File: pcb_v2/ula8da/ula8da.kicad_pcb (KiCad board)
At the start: 2 copper layers, 66.6 x 123.8 mm, 28 parts, among them J1 addr_decoder, J2 Conn_01x07, J3 Conn_01x07, J4 Conn_01x07, J5 Conn_01x07, Q1 BC548, U1 74LS138, U2 74HC238, U3 74HC238, U4 74HC238, U5 74LS04, U6 74LS244, U7 74LS04, U8 MC14495P, U9 SA39-11EWA

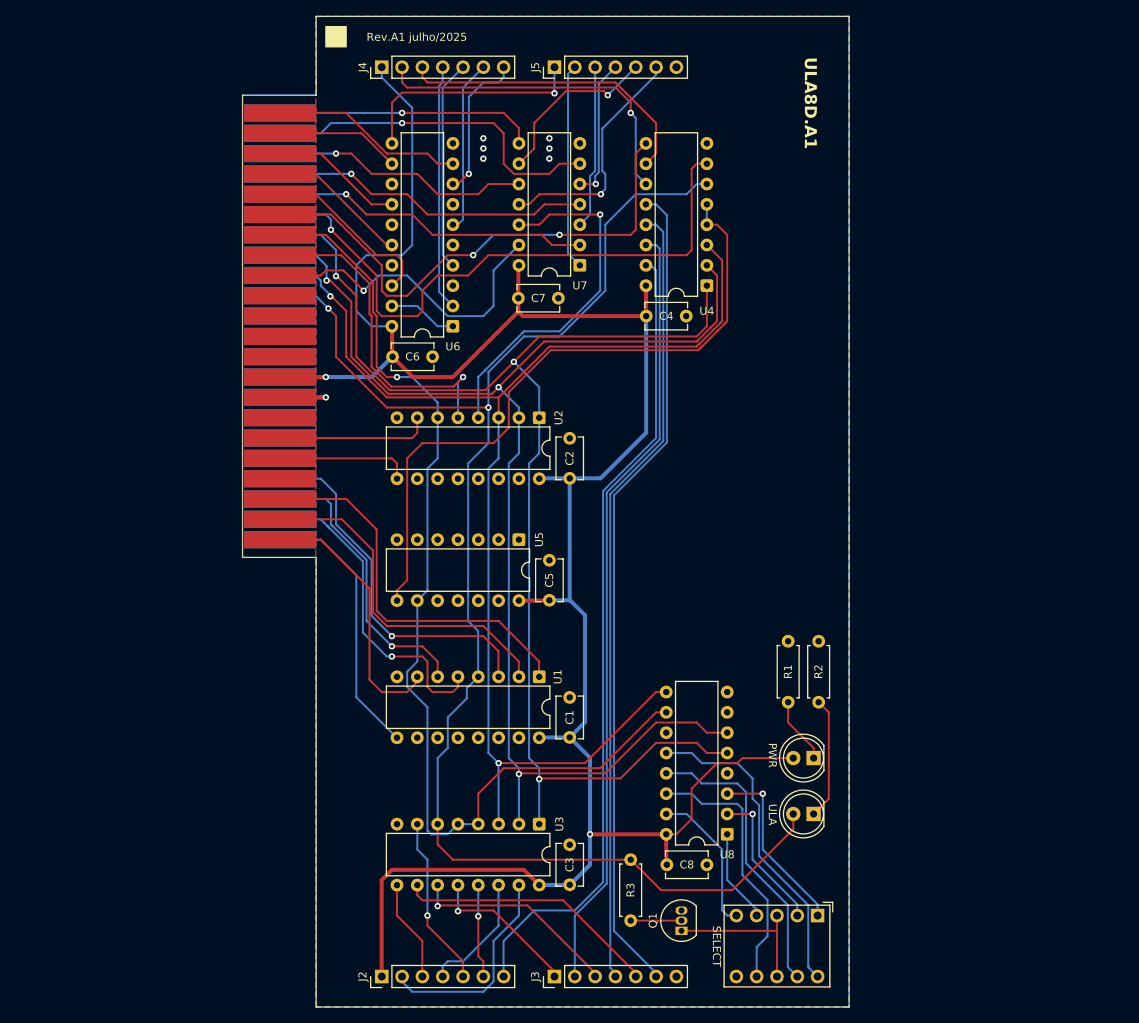
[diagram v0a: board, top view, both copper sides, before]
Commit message: PCB concluída
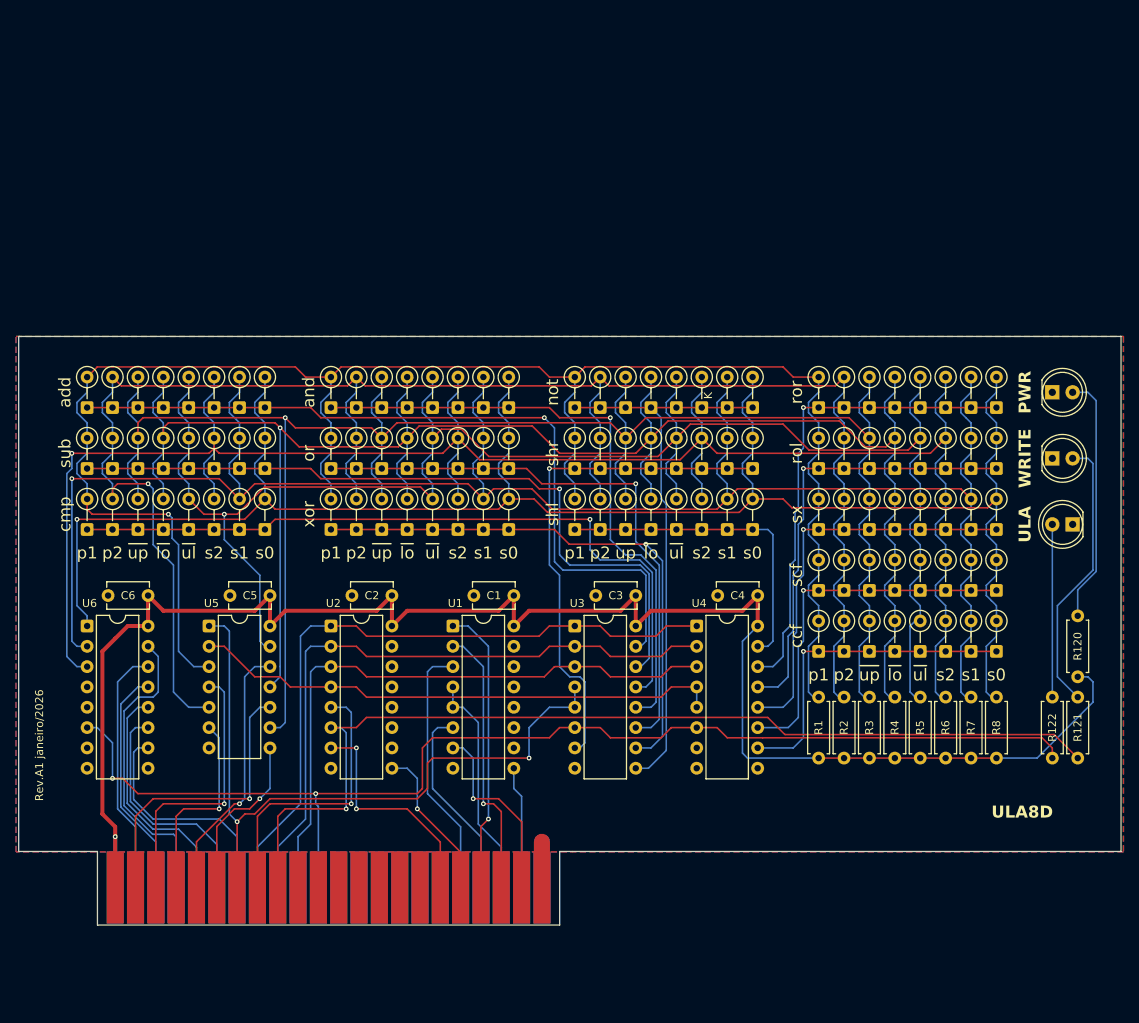
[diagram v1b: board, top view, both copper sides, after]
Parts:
- removed C7, C8: 100nF, Capacitor_THT:C_Disc_D5.1mm_W3.2mm_P5.00mm
- removed J2, J3, J4, J5: Conn_01x07, Connector_PinHeader_2.54mm:PinHeader_1x07_P2.54mm_Vertical
- removed Q1: BC548, Package_TO_SOT_THT:TO-92_Inline
- removed U7: 74LS04, Package_DIP:DIP-14_W7.62mm
- removed U8: MC14495P, Package_DIP:DIP-16_W7.62mm
- removed U9: SA39-11EWA, Display_7Segment:Sx39-1xxxxx
- added D10: 1N4148, Diode_THT:D_DO-35_SOD27_P3.81mm_Vertical_KathodeUp, F.Cu at (45.1, 88.9)
- added D100: 1N4148, Diode_THT:D_DO-35_SOD27_P3.81mm_Vertical_KathodeUp, F.Cu at (142.9, 104.1)
- added D101: 1N4148, Diode_THT:D_DO-35_SOD27_P3.81mm_Vertical_KathodeUp, F.Cu at (146.1, 104.1)
- added D102: 1N4148, Diode_THT:D_DO-35_SOD27_P3.81mm_Vertical_KathodeUp, F.Cu at (149.2, 104.1)
- added D103: 1N4148, Diode_THT:D_DO-35_SOD27_P3.81mm_Vertical_KathodeUp, F.Cu at (152.4, 104.1)
- added D104: 1N4148, Diode_THT:D_DO-35_SOD27_P3.81mm_Vertical_KathodeUp, F.Cu at (155.6, 104.1)
- added D105: 1N4148, Diode_THT:D_DO-35_SOD27_P3.81mm_Vertical_KathodeUp, F.Cu at (133.3, 111.8)
- added D106: 1N4148, Diode_THT:D_DO-35_SOD27_P3.81mm_Vertical_KathodeUp, F.Cu at (136.5, 111.8)
- added D107: 1N4148, Diode_THT:D_DO-35_SOD27_P3.81mm_Vertical_KathodeUp, F.Cu at (139.7, 111.8)
- added D108: 1N4148, Diode_THT:D_DO-35_SOD27_P3.81mm_Vertical_KathodeUp, F.Cu at (142.9, 111.8)
- added D109: 1N4148, Diode_THT:D_DO-35_SOD27_P3.81mm_Vertical_KathodeUp, F.Cu at (146.1, 111.8)
- added D11: 1N4148, Diode_THT:D_DO-35_SOD27_P3.81mm_Vertical_KathodeUp, F.Cu at (48.3, 88.9)
- added D110: 1N4148, Diode_THT:D_DO-35_SOD27_P3.81mm_Vertical_KathodeUp, F.Cu at (149.2, 111.8)
- added D111: 1N4148, Diode_THT:D_DO-35_SOD27_P3.81mm_Vertical_KathodeUp, F.Cu at (152.4, 111.8)
- added D112: 1N4148, Diode_THT:D_DO-35_SOD27_P3.81mm_Vertical_KathodeUp, F.Cu at (155.6, 111.8)
- added D12: 1N4148, Diode_THT:D_DO-35_SOD27_P3.81mm_Vertical_KathodeUp, F.Cu at (51.4, 88.9)
- added D120: LED, LED_THT:LED_D5.0mm, F.Cu at (162.6, 79.4)
- added D121: LED, LED_THT:LED_D5.0mm, F.Cu at (162.6, 87.6)
- added D122: LED, LED_THT:LED_D5.0mm, F.Cu at (165.1, 95.9)
- added D13: 1N4148, Diode_THT:D_DO-35_SOD27_P3.81mm_Vertical_KathodeUp, F.Cu at (54.6, 88.9)
- added D14: 1N4148, Diode_THT:D_DO-35_SOD27_P3.81mm_Vertical_KathodeUp, F.Cu at (57.8, 88.9)
- added D15: 1N4148, Diode_THT:D_DO-35_SOD27_P3.81mm_Vertical_KathodeUp, F.Cu at (61.0, 88.9)
- added D16: 1N4148, Diode_THT:D_DO-35_SOD27_P3.81mm_Vertical_KathodeUp, F.Cu at (64.1, 88.9)
- added D17: 1N4148, Diode_THT:D_DO-35_SOD27_P3.81mm_Vertical_KathodeUp, F.Cu at (41.9, 96.5)
- added D18: 1N4148, Diode_THT:D_DO-35_SOD27_P3.81mm_Vertical_KathodeUp, F.Cu at (45.1, 96.5)
- added D19: 1N4148, Diode_THT:D_DO-35_SOD27_P3.81mm_Vertical_KathodeUp, F.Cu at (48.3, 96.5)
- added D20: 1N4148, Diode_THT:D_DO-35_SOD27_P3.81mm_Vertical_KathodeUp, F.Cu at (51.4, 96.5)
- added D21: 1N4148, Diode_THT:D_DO-35_SOD27_P3.81mm_Vertical_KathodeUp, F.Cu at (54.6, 96.5)
- added D22: 1N4148, Diode_THT:D_DO-35_SOD27_P3.81mm_Vertical_KathodeUp, F.Cu at (57.8, 96.5)
- added D23: 1N4148, Diode_THT:D_DO-35_SOD27_P3.81mm_Vertical_KathodeUp, F.Cu at (61.0, 96.5)
- added D24: 1N4148, Diode_THT:D_DO-35_SOD27_P3.81mm_Vertical_KathodeUp, F.Cu at (64.1, 96.5)
- added D25: 1N4148, Diode_THT:D_DO-35_SOD27_P3.81mm_Vertical_KathodeUp, F.Cu at (72.4, 81.3)
- added D26: 1N4148, Diode_THT:D_DO-35_SOD27_P3.81mm_Vertical_KathodeUp, F.Cu at (75.6, 81.3)
- added D27: 1N4148, Diode_THT:D_DO-35_SOD27_P3.81mm_Vertical_KathodeUp, F.Cu at (78.7, 81.3)
- added D28: 1N4148, Diode_THT:D_DO-35_SOD27_P3.81mm_Vertical_KathodeUp, F.Cu at (81.9, 81.3)
- added D29: 1N4148, Diode_THT:D_DO-35_SOD27_P3.81mm_Vertical_KathodeUp, F.Cu at (85.1, 81.3)
- added D3: 1N4148, Diode_THT:D_DO-35_SOD27_P3.81mm_Vertical_KathodeUp, F.Cu at (48.3, 81.3)
- added D30: 1N4148, Diode_THT:D_DO-35_SOD27_P3.81mm_Vertical_KathodeUp, F.Cu at (88.3, 81.3)
- added D31: 1N4148, Diode_THT:D_DO-35_SOD27_P3.81mm_Vertical_KathodeUp, F.Cu at (91.4, 81.3)
- added D32: 1N4148, Diode_THT:D_DO-35_SOD27_P3.81mm_Vertical_KathodeUp, F.Cu at (94.6, 81.3)
- added D33: 1N4148, Diode_THT:D_DO-35_SOD27_P3.81mm_Vertical_KathodeUp, F.Cu at (72.4, 88.9)
- added D34: 1N4148, Diode_THT:D_DO-35_SOD27_P3.81mm_Vertical_KathodeUp, F.Cu at (75.6, 88.9)
- added D35: 1N4148, Diode_THT:D_DO-35_SOD27_P3.81mm_Vertical_KathodeUp, F.Cu at (78.7, 88.9)
- added D36: 1N4148, Diode_THT:D_DO-35_SOD27_P3.81mm_Vertical_KathodeUp, F.Cu at (81.9, 88.9)
- added D37: 1N4148, Diode_THT:D_DO-35_SOD27_P3.81mm_Vertical_KathodeUp, F.Cu at (85.1, 88.9)
- added D38: 1N4148, Diode_THT:D_DO-35_SOD27_P3.81mm_Vertical_KathodeUp, F.Cu at (88.3, 88.9)
- added D39: 1N4148, Diode_THT:D_DO-35_SOD27_P3.81mm_Vertical_KathodeUp, F.Cu at (91.4, 88.9)
- added D4: 1N4148, Diode_THT:D_DO-35_SOD27_P3.81mm_Vertical_KathodeUp, F.Cu at (51.4, 81.3)
- added D40: 1N4148, Diode_THT:D_DO-35_SOD27_P3.81mm_Vertical_KathodeUp, F.Cu at (94.6, 88.9)
- added D41: 1N4148, Diode_THT:D_DO-35_SOD27_P3.81mm_Vertical_KathodeUp, F.Cu at (72.4, 96.5)
- added D42: 1N4148, Diode_THT:D_DO-35_SOD27_P3.81mm_Vertical_KathodeUp, F.Cu at (75.6, 96.5)
- added D43: 1N4148, Diode_THT:D_DO-35_SOD27_P3.81mm_Vertical_KathodeUp, F.Cu at (78.7, 96.5)
- added D44: 1N4148, Diode_THT:D_DO-35_SOD27_P3.81mm_Vertical_KathodeUp, F.Cu at (81.9, 96.5)
- added D45: 1N4148, Diode_THT:D_DO-35_SOD27_P3.81mm_Vertical_KathodeUp, F.Cu at (85.1, 96.5)
- added D46: 1N4148, Diode_THT:D_DO-35_SOD27_P3.81mm_Vertical_KathodeUp, F.Cu at (88.3, 96.5)
- added D47: 1N4148, Diode_THT:D_DO-35_SOD27_P3.81mm_Vertical_KathodeUp, F.Cu at (91.4, 96.5)
- added D48: 1N4148, Diode_THT:D_DO-35_SOD27_P3.81mm_Vertical_KathodeUp, F.Cu at (94.6, 96.5)
- added D49: 1N4148, Diode_THT:D_DO-35_SOD27_P3.81mm_Vertical_KathodeUp, F.Cu at (102.9, 81.3)
- added D5: 1N4148, Diode_THT:D_DO-35_SOD27_P3.81mm_Vertical_KathodeUp, F.Cu at (54.6, 81.3)
- added D50: 1N4148, Diode_THT:D_DO-35_SOD27_P3.81mm_Vertical_KathodeUp, F.Cu at (106.0, 81.3)
- added D51: 1N4148, Diode_THT:D_DO-35_SOD27_P3.81mm_Vertical_KathodeUp, F.Cu at (109.2, 81.3)
- added D52: 1N4148, Diode_THT:D_DO-35_SOD27_P3.81mm_Vertical_KathodeUp, F.Cu at (112.4, 81.3)
- added D53: 1N4148, Diode_THT:D_DO-35_SOD27_P3.81mm_Vertical_KathodeUp, F.Cu at (115.6, 81.3)
- added D54: 1N4148, Diode_THT:D_DO-35_SOD27_P3.81mm_Vertical_KathodeUp, F.Cu at (118.7, 81.3)
- added D55: 1N4148, Diode_THT:D_DO-35_SOD27_P3.81mm_Vertical_KathodeUp, F.Cu at (121.9, 81.3)
- added D56: 1N4148, Diode_THT:D_DO-35_SOD27_P3.81mm_Vertical_KathodeUp, F.Cu at (125.1, 81.3)
- added D57: 1N4148, Diode_THT:D_DO-35_SOD27_P3.81mm_Vertical_KathodeUp, F.Cu at (102.9, 88.9)
- added D58: 1N4148, Diode_THT:D_DO-35_SOD27_P3.81mm_Vertical_KathodeUp, F.Cu at (106.0, 88.9)
- added D59: 1N4148, Diode_THT:D_DO-35_SOD27_P3.81mm_Vertical_KathodeUp, F.Cu at (109.2, 88.9)
- added D6: 1N4148, Diode_THT:D_DO-35_SOD27_P3.81mm_Vertical_KathodeUp, F.Cu at (57.8, 81.3)
- added D60: 1N4148, Diode_THT:D_DO-35_SOD27_P3.81mm_Vertical_KathodeUp, F.Cu at (112.4, 88.9)
- added D61: 1N4148, Diode_THT:D_DO-35_SOD27_P3.81mm_Vertical_KathodeUp, F.Cu at (115.6, 88.9)
- added D62: 1N4148, Diode_THT:D_DO-35_SOD27_P3.81mm_Vertical_KathodeUp, F.Cu at (118.7, 88.9)
- added D63: 1N4148, Diode_THT:D_DO-35_SOD27_P3.81mm_Vertical_KathodeUp, F.Cu at (121.9, 88.9)
- added D64: 1N4148, Diode_THT:D_DO-35_SOD27_P3.81mm_Vertical_KathodeUp, F.Cu at (125.1, 88.9)
- added D65: 1N4148, Diode_THT:D_DO-35_SOD27_P3.81mm_Vertical_KathodeUp, F.Cu at (102.9, 96.5)
- added D66: 1N4148, Diode_THT:D_DO-35_SOD27_P3.81mm_Vertical_KathodeUp, F.Cu at (106.0, 96.5)
- added D67: 1N4148, Diode_THT:D_DO-35_SOD27_P3.81mm_Vertical_KathodeUp, F.Cu at (109.2, 96.5)
- added D68: 1N4148, Diode_THT:D_DO-35_SOD27_P3.81mm_Vertical_KathodeUp, F.Cu at (112.4, 96.5)
- added D69: 1N4148, Diode_THT:D_DO-35_SOD27_P3.81mm_Vertical_KathodeUp, F.Cu at (115.6, 96.5)
- added D7: 1N4148, Diode_THT:D_DO-35_SOD27_P3.81mm_Vertical_KathodeUp, F.Cu at (61.0, 81.3)
- added D70: 1N4148, Diode_THT:D_DO-35_SOD27_P3.81mm_Vertical_KathodeUp, F.Cu at (118.7, 96.5)
- added D71: 1N4148, Diode_THT:D_DO-35_SOD27_P3.81mm_Vertical_KathodeUp, F.Cu at (121.9, 96.5)
- added D72: 1N4148, Diode_THT:D_DO-35_SOD27_P3.81mm_Vertical_KathodeUp, F.Cu at (125.1, 96.5)
- added D73: 1N4148, Diode_THT:D_DO-35_SOD27_P3.81mm_Vertical_KathodeUp, F.Cu at (133.3, 81.3)
- added D74: 1N4148, Diode_THT:D_DO-35_SOD27_P3.81mm_Vertical_KathodeUp, F.Cu at (136.5, 81.3)
- added D75: 1N4148, Diode_THT:D_DO-35_SOD27_P3.81mm_Vertical_KathodeUp, F.Cu at (139.7, 81.3)
- added D76: 1N4148, Diode_THT:D_DO-35_SOD27_P3.81mm_Vertical_KathodeUp, F.Cu at (142.9, 81.3)
- added D77: 1N4148, Diode_THT:D_DO-35_SOD27_P3.81mm_Vertical_KathodeUp, F.Cu at (146.1, 81.3)
- added D78: 1N4148, Diode_THT:D_DO-35_SOD27_P3.81mm_Vertical_KathodeUp, F.Cu at (149.2, 81.3)
- added D79: 1N4148, Diode_THT:D_DO-35_SOD27_P3.81mm_Vertical_KathodeUp, F.Cu at (152.4, 81.3)
- added D8: 1N4148, Diode_THT:D_DO-35_SOD27_P3.81mm_Vertical_KathodeUp, F.Cu at (64.1, 81.3)
- added D80: 1N4148, Diode_THT:D_DO-35_SOD27_P3.81mm_Vertical_KathodeUp, F.Cu at (155.6, 81.3)
- added D81: 1N4148, Diode_THT:D_DO-35_SOD27_P3.81mm_Vertical_KathodeUp, F.Cu at (133.3, 88.9)
- added D82: 1N4148, Diode_THT:D_DO-35_SOD27_P3.81mm_Vertical_KathodeUp, F.Cu at (136.5, 88.9)
- added D83: 1N4148, Diode_THT:D_DO-35_SOD27_P3.81mm_Vertical_KathodeUp, F.Cu at (139.7, 88.9)
- added D84: 1N4148, Diode_THT:D_DO-35_SOD27_P3.81mm_Vertical_KathodeUp, F.Cu at (142.9, 88.9)
- added D85: 1N4148, Diode_THT:D_DO-35_SOD27_P3.81mm_Vertical_KathodeUp, F.Cu at (146.1, 88.9)
- added D86: 1N4148, Diode_THT:D_DO-35_SOD27_P3.81mm_Vertical_KathodeUp, F.Cu at (149.2, 88.9)
- added D87: 1N4148, Diode_THT:D_DO-35_SOD27_P3.81mm_Vertical_KathodeUp, F.Cu at (152.4, 88.9)
- added D88: 1N4148, Diode_THT:D_DO-35_SOD27_P3.81mm_Vertical_KathodeUp, F.Cu at (155.6, 88.9)
- added D89: 1N4148, Diode_THT:D_DO-35_SOD27_P3.81mm_Vertical_KathodeUp, F.Cu at (133.3, 96.5)
- added D9: 1N4148, Diode_THT:D_DO-35_SOD27_P3.81mm_Vertical_KathodeUp, F.Cu at (41.9, 88.9)
- added D90: 1N4148, Diode_THT:D_DO-35_SOD27_P3.81mm_Vertical_KathodeUp, F.Cu at (136.5, 96.5)
- added D91: 1N4148, Diode_THT:D_DO-35_SOD27_P3.81mm_Vertical_KathodeUp, F.Cu at (139.7, 96.5)
- added D92: 1N4148, Diode_THT:D_DO-35_SOD27_P3.81mm_Vertical_KathodeUp, F.Cu at (142.9, 96.5)
- added D93: 1N4148, Diode_THT:D_DO-35_SOD27_P3.81mm_Vertical_KathodeUp, F.Cu at (146.1, 96.5)
- added D94: 1N4148, Diode_THT:D_DO-35_SOD27_P3.81mm_Vertical_KathodeUp, F.Cu at (149.2, 96.5)
- added D95: 1N4148, Diode_THT:D_DO-35_SOD27_P3.81mm_Vertical_KathodeUp, F.Cu at (152.4, 96.5)
- added D96: 1N4148, Diode_THT:D_DO-35_SOD27_P3.81mm_Vertical_KathodeUp, F.Cu at (155.6, 96.5)
- added D97: 1N4148, Diode_THT:D_DO-35_SOD27_P3.81mm_Vertical_KathodeUp, F.Cu at (133.3, 104.1)
- added D98: 1N4148, Diode_THT:D_DO-35_SOD27_P3.81mm_Vertical_KathodeUp, F.Cu at (136.5, 104.1)
- added D99: 1N4148, Diode_THT:D_DO-35_SOD27_P3.81mm_Vertical_KathodeUp, F.Cu at (139.7, 104.1)
- added R120: 1K, Resistor_THT:R_Axial_DIN0207_L6.3mm_D2.5mm_P7.62mm_Horizontal, F.Cu at (165.7, 114.9)
- added R121: 1K, Resistor_THT:R_Axial_DIN0207_L6.3mm_D2.5mm_P7.62mm_Horizontal, F.Cu at (165.7, 125.1)
- added R122: 1K, Resistor_THT:R_Axial_DIN0207_L6.3mm_D2.5mm_P7.62mm_Horizontal, F.Cu at (162.6, 125.1)
- added R4: 10K, Resistor_THT:R_Axial_DIN0207_L6.3mm_D2.5mm_P7.62mm_Horizontal, F.Cu at (142.9, 117.5)
- added R5: 10K, Resistor_THT:R_Axial_DIN0207_L6.3mm_D2.5mm_P7.62mm_Horizontal, F.Cu at (146.1, 117.5)
- added R6: 10K, Resistor_THT:R_Axial_DIN0207_L6.3mm_D2.5mm_P7.62mm_Horizontal, F.Cu at (149.2, 117.5)
- added R7: 10K, Resistor_THT:R_Axial_DIN0207_L6.3mm_D2.5mm_P7.62mm_Horizontal, F.Cu at (152.4, 117.5)
- added R8: 10K, Resistor_THT:R_Axial_DIN0207_L6.3mm_D2.5mm_P7.62mm_Horizontal, F.Cu at (155.6, 117.5)
- D1, D2: value LED -> 1N4148; footprint LED_THT:LED_D5.0mm -> Diode_THT:D_DO-35_SOD27_P3.81mm_Vertical_KathodeUp
- R1, R2: value 1K -> 10K
- U3, U4: value 74HC238 -> 74LS138
- U6: value 74LS244 -> 74LS138; footprint Package_DIP:DIP-20_W7.62mm -> Package_DIP:DIP-16_W7.62mm
- moved D2 101.3 mm to (45.1, 81.3), turned to 90 degrees
- moved D1 100.8 mm to (41.9, 81.3), turned to 90 degrees
- moved J1 99.0 mm to (45.4, 141.3), turned to 90 degrees
- moved U6 59.1 mm to (41.9, 108.6), turned to 0 degrees
- moved C6 46.4 mm to (44.5, 104.8)
- moved U4 42.6 mm to (118.1, 108.6), turned to 0 degrees
- moved R3 40.9 mm to (139.7, 117.5), turned to -90 degrees
- moved U5 40.2 mm to (57.1, 108.6), turned to 0 degrees
- moved C5 40.2 mm to (59.8, 104.8), turned to 0 degrees
- moved U2 36.8 mm to (72.4, 108.6), turned to 0 degrees
- moved C4 35.1 mm to (120.7, 104.8), turned to 0 degrees
- moved C2 33.6 mm to (75.0, 104.8), turned to 0 degrees
- moved C3 31.3 mm to (105.5, 104.8), turned to 0 degrees
- moved U3 25.2 mm to (102.9, 108.6), turned to 0 degrees
- moved C1 17.5 mm to (90.2, 104.8), turned to 0 degrees
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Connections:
- C6 pad 1: +5V -> GND
- C6 pad 2: GND -> +5V
- D1 pad 1: Net-(D1-K) -> ~{do_add}
- D1 pad 2: +5V -> Net-(D1-A)
- D2 pad 1: Net-(D2-K) -> ~{do_add}
- D2 pad 2: ula_enable -> Net-(D10-A)
- J1 pad 1: invert_lower_bus -> +5V
- J1 pad 14: +5V -> unconnected-(J1-Pin_14-Pad14)
- J1 pad 15: GND -> unconnected-(J1-Pin_15-Pad15)
- J1 pad 19: unconnected-(J1-Pin_19-Pad19) -> rd_addr_0
- J1 pad 2: rotate/clear -> invert_lower_bus
- J1 pad 20: rd_addr_0 -> rd_addr_1
- J1 pad 21: rd_addr_1 -> ~{read_acc}
- J1 pad 22: ~{read_acc} -> GND
- J1 pad 23: ~{select_bitwise} -> +5V
- J1 pad 24: ~{select_xor} -> ~{select_bitwise}
- J1 pad 25: ~{select_adder} -> ~{select_xor}
- J1 pad 26: ~{select_shifter} -> ~{select_adder}
- J1 pad 27: ~{select_sx} -> ~{select_shifter}
- J1 pad 28: clrif -> ~{select_sx}
- J1 pad 29: wr_addr_0 -> ~{select_cf}
- J1 pad 3: right/set -> rotate/value
- J1 pad 30: wr_addr_1 -> wr_addr_0
- J1 pad 31: wr_addr_2 -> wr_addr_1
- J1 pad 32: ula_enable -> wr_addr_2
- J1 pad 33: unconnected-(J1-Pin_33-Pad33) -> ula_enable
- J1 pad 36: +5V -> unconnected-(J1-Pin_36-Pad36)
- J1 pad 37: GND -> unconnected-(J1-Pin_37-Pad37)
- J1 pad 4: invert_ula_bus -> right/mode
- J1 pad 40: unconnected-(J1-Pin_40-Pad40) -> rd_addr_2
- J1 pad 41: rd_addr_2 -> rd_addr_3
- J1 pad 42: rd_addr_3 -> rd_addr_4
- J1 pad 43: rd_addr_4 -> ~{read_psw}
- J1 pad 44: ~{read_psw} -> GND
- J1 pad 5: invert_upper_bus -> invert_ula_bus
- J1 pad 6: setif -> invert_upper_bus
- J1 pad 9: write_clock -> write_enable
- R1 pad 1: Net-(D1-K) -> Net-(D1-A)
- R1 pad 2: GND -> +5V
- R2 pad 1: Net-(D2-K) -> Net-(D10-A)
- R2 pad 2: GND -> +5V
- R3 pad 1: Net-(Q1-B) -> Net-(D107-A)
- R3 pad 2: ula_enable -> +5V
- U1 pad 4: ula_enable -> rd_addr_4
- U2 pad 4: Net-(U2-~{E1}) -> ~{wr_addr_3}
- U2 pad 6: wr_addr_3 -> write_enable
- U3 pad 10: do_xor -> ~{do_xor}
- U3 pad 11: do_or -> ~{do_or}
- U3 pad 12: do_and -> ~{do_and}
- U3 pad 13: do_cmp -> ~{do_cmp}
- U3 pad 14: do_sub -> ~{do_sub}
- U3 pad 15: do_add -> ~{do_add}
- U3 pad 7: do_shr -> ~{do_shr}
- U3 pad 9: do_not -> ~{do_not}
- U4 pad 10: do_clrcf -> ~{do_clrcf}
- U4 pad 11: do_setcf -> ~{do_setcf}
- U4 pad 12: do_sx -> ~{do_sx}
- U4 pad 13: do_rol -> ~{do_rol}
- U4 pad 14: do_ror -> ~{do_ror}
- U4 pad 15: do_shl -> ~{do_shl}
- U4 pad 4: Net-(U4-~{E1}) -> ~{wr_addr_3}
- U4 pad 5: Net-(U4-~{E1}) -> ~{wr_addr_3}
- U4 pad 7: clrif -> unconnected-(U4-O7-Pad7)
- U4 pad 9: setif -> unconnected-(U4-O6-Pad9)
- U5 pad 1: unconnected-(U5-Pad1) -> wr_addr_3
- U5 pad 10: unconnected-(U5-Pad10) -> invert_lower_bus
- U5 pad 11: unconnected-(U5-Pad11) -> Net-(D100-A)
- U5 pad 12: unconnected-(U5-Pad12) -> invert_ula_bus
- U5 pad 13: unconnected-(U5-Pad13) -> Net-(D101-A)
- U5 pad 2: unconnected-(U5-Pad2) -> ~{wr_addr_3}
- U5 pad 3: unconnected-(U5-Pad3) -> Net-(D1-A)
- U5 pad 4: unconnected-(U5-Pad4) -> rotate/value
- U5 pad 5: unconnected-(U5-Pad5) -> Net-(D10-A)
- U5 pad 6: unconnected-(U5-Pad6) -> right/mode
- U5 pad 8: Net-(U4-~{E1}) -> invert_upper_bus
- U5 pad 9: wr_addr_3 -> Net-(D107-A)
- U6 pad 1: GND -> Net-(D104-A)
- U6 pad 10: GND -> ~{select_cf}
- U6 pad 11: Net-(J5-Pin_1) -> ~{select_sx}
- U6 pad 12: rotate/clear -> ~{select_shifter}
- U6 pad 13: unconnected-(U6-I1b-Pad13) -> ~{select_xor}
- U6 pad 14: right/set -> ~{select_bitwise}
- U6 pad 15: unconnected-(U6-I2b-Pad15) -> ~{select_adder}
- U6 pad 16: invert_ula_bus -> +5V
- U6 pad 3: unconnected-(U6-O3b-Pad3) -> Net-(D102-A)
- U6 pad 4: Net-(J4-Pin_5) -> GND
- U6 pad 5: unconnected-(U6-O2b-Pad5) -> GND
- U6 pad 6: Net-(J4-Pin_6) -> ula_enable
- U6 pad 8: Net-(J4-Pin_7) -> GND
- U6 pad 9: invert_lower_bus -> unconnected-(U6-O6-Pad9)
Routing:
- net Net-(D102-A): track 0.00 -> 241.0 mm, vias 0 -> 1
- net Net-(D107-A): track 0.00 -> 237.1 mm, vias 0 -> 1
- net Net-(D104-A): track 0.00 -> 231.3 mm, vias 0 -> 1
- net Net-(D10-A): track 0.00 -> 230.3 mm, vias 0 -> 1
- net Net-(D100-A): track 0.00 -> 228.7 mm, vias 0 -> 1
- net Net-(D1-A): track 0.00 -> 227.1 mm, vias 0 -> 1
- net Net-(D101-A): track 0.00 -> 214.8 mm, vias 0 -> 1
- net Net-(D103-A): track 30.7 -> 238.2 mm, vias 0 -> 1
- net write_enable: track 0.00 -> 125.5 mm, vias 0 -> 1
- net do_sx: track 102.8 -> 0.00 mm
- net do_shl: track 100.2 -> 0.00 mm
- net ~{do_add}: track 0.00 -> 98.4 mm, vias 0 -> 1
- net do_rol: track 98.2 -> 0.00 mm
- net do_ror: track 96.9 -> 0.00 mm
- net ~{do_sub}: track 0.00 -> 93.2 mm, vias 0 -> 1
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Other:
- board size 66.6 x 123.8 mm -> 137.8 x 64.4 mm
- board text added: "Rev.A1 janeiro/2026"
- board text added: "ULA8D"
- board text added: "WRITE"
- board text added: "add"
- board text added: "and"
- board text added: "ccf"
- board text added: "cmp"
- board text added: "not"
- board text added: "or"
- board text added: "p1"
- board text added: "p2"
- board text added: "rol"
- board text added: "ror"
- board text added: "s0"
- board text added: "s1"
- board text added: "s2"
- board text added: "scf"
- board text added: "shl"
- board text added: "shr"
- board text added: "sub"
- board text added: "sx"
- board text added: "xor"
- board text added: "~{lo}"
- board text added: "~{ul}"
- board text added: "~{up}"
- board text removed: "Rev.A1 julho/2025"
- board text removed: "SELECT"
- board text removed: "ULA8D.A1"
